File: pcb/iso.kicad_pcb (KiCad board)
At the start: 2 copper layers, 27.5 x 40.3 mm, 19 parts, among them J1 Conn_01x06, U1 ATmega328P-AU, U2 SRV05-4, X1 Crystal_GND24_Small

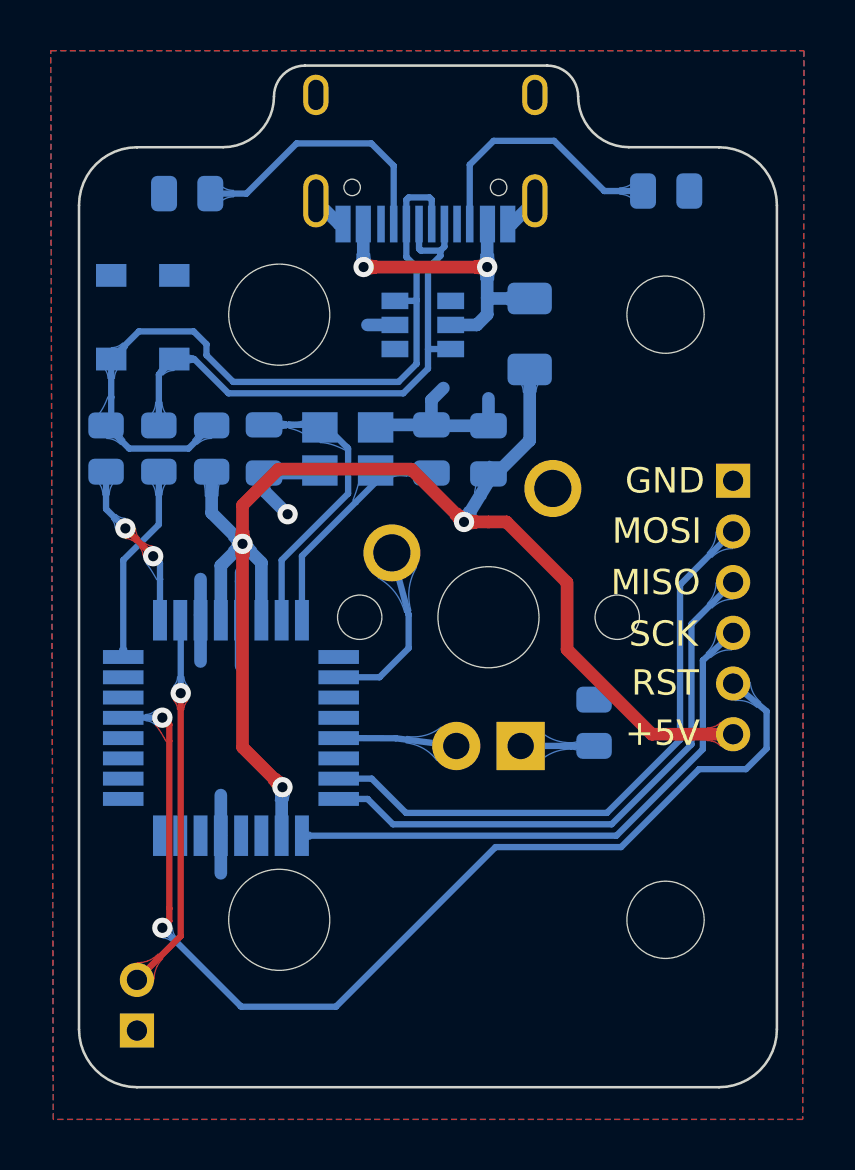
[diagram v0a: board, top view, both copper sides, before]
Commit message: RGB!!!
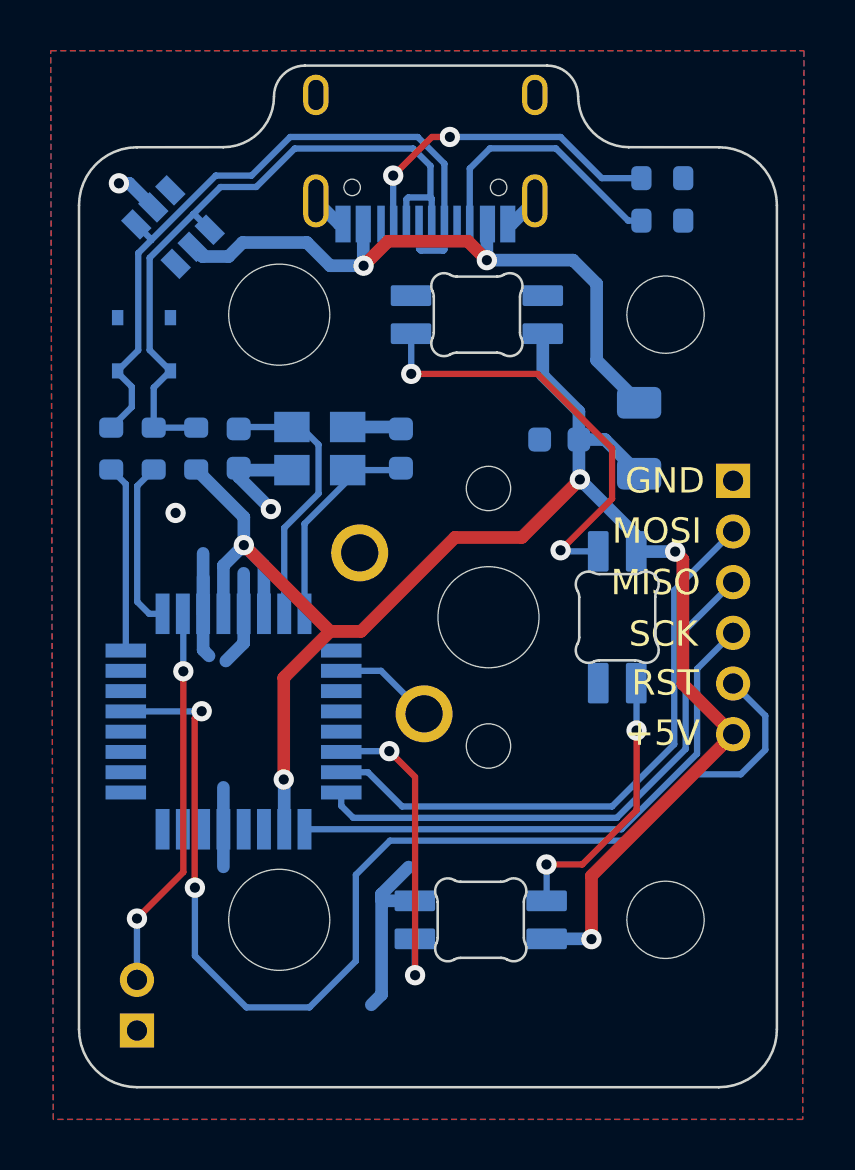
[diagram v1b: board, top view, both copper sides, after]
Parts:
- removed R7: 1k, Resistor_SMD:R_0805_2012Metric
- added LED1: SK6812MINI, custom_parts:SK6812MINIE-simple, F.Cu at (157.1, 96.0)
- added LED2: SK6812MINI, custom_parts:SK6812MINIE-simple, F.Cu at (162.5, 84.0)
- added LED3: SK6812MINI, custom_parts:SK6812MINIE-simple, F.Cu at (157.0, 72.1)
- C1, C7, C8: footprint Capacitor_SMD:C_0805_2012Metric -> Capacitor_SMD:C_0603_1608Metric
- D1, D2: footprint Diode_SMD:D_SOD-123 -> Diode_SMD:D_SOD-323
- MX1: value MX-LED -> MX-NoLED; footprint MX_Only:MXOnly-ISO-ReversedStabilizers -> custom_parts:MXOnly-ISO-ROTATEDCCW-ReversedStabilizers-NoLED
- R1, R2, R3, R4, R5: footprint Resistor_SMD:R_0805_2012Metric -> Resistor_SMD:R_0603_1608Metric
- moved R1 18.8 mm to (164.3, 66.7), turned to 180 degrees
- moved U2 10.6 mm to (145.0, 68.6), turned to 315 degrees
- moved F1 5.96 mm to (163.4, 77.0)
- moved C1 2.82 mm to (160.2, 77.0), turned to 180 degrees
- moved D1 2.57 mm to (144.9, 73.3)
- moved D2 2.48 mm to (142.8, 73.3)
- moved R4 1.88 mm to (144.2, 77.4)
- moved R5 1.88 mm to (142.5, 77.4)
- moved C7 1.20 mm to (154.0, 77.4)
- moved R2 1.18 mm to (164.3, 68.4)
- moved X1 1.10 mm to (150.8, 77.4)
- moved C8 1.00 mm to (147.6, 77.4)
- moved R3 0.61 mm to (145.9, 77.4)
- moved U1 0.27 mm to (147.4, 88.1)
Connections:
- U1 pad 13: LED -> Net-(U1-Pad13)
- U1 pad 14: Net-(U1-Pad14) -> LED
- U2 pad 1: Net-(U2-Pad1) -> Net-(D2-Pad1)
- U2 pad 3: Net-(D1-Pad1) -> Net-(U2-Pad3)
- U2 pad 4: Net-(U2-Pad4) -> Net-(D1-Pad1)
- U2 pad 6: Net-(D2-Pad1) -> Net-(U2-Pad6)
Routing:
- net Net-(LED2-Pad1): track 0.00 -> 17.1 mm, vias 0 -> 2
- net +5V: track 56.2 -> 70.5 mm, vias 3 -> 5
- net VCC: track 13.4 -> 26.3 mm
- net Net-(LED1-Pad1): track 0.00 -> 10.9 mm, vias 0 -> 2
- net LED: track 4.66 -> 12.6 mm, vias 0 -> 2
- net Net-(D2-Pad1): track 22.6 -> 28.5 mm
- net GND: track 25.9 -> 31.1 mm, vias 1 -> 3
- net Net-(D1-Pad1): track 31.0 -> 27.3 mm
- net SW: track 7.08 -> 3.97 mm
- net Net-(MX1-Pad4): track 2.90 -> 0.00 mm
- net RESET: track 42.6 -> 45.5 mm
- net Net-(R1-Pad2): track 10.7 -> 13.0 mm, vias 0 -> 2
- net Net-(C7-Pad1): track 9.68 -> 8.51 mm
- net Net-(C8-Pad1): track 11.6 -> 10.7 mm
- net D+: track 7.93 -> 7.38 mm
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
